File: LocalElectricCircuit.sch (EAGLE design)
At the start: 49 parts, among them IC1 PIC32MX360F512L, U1 ADS1118, U2 ADS1118, X2 MALE_VGA

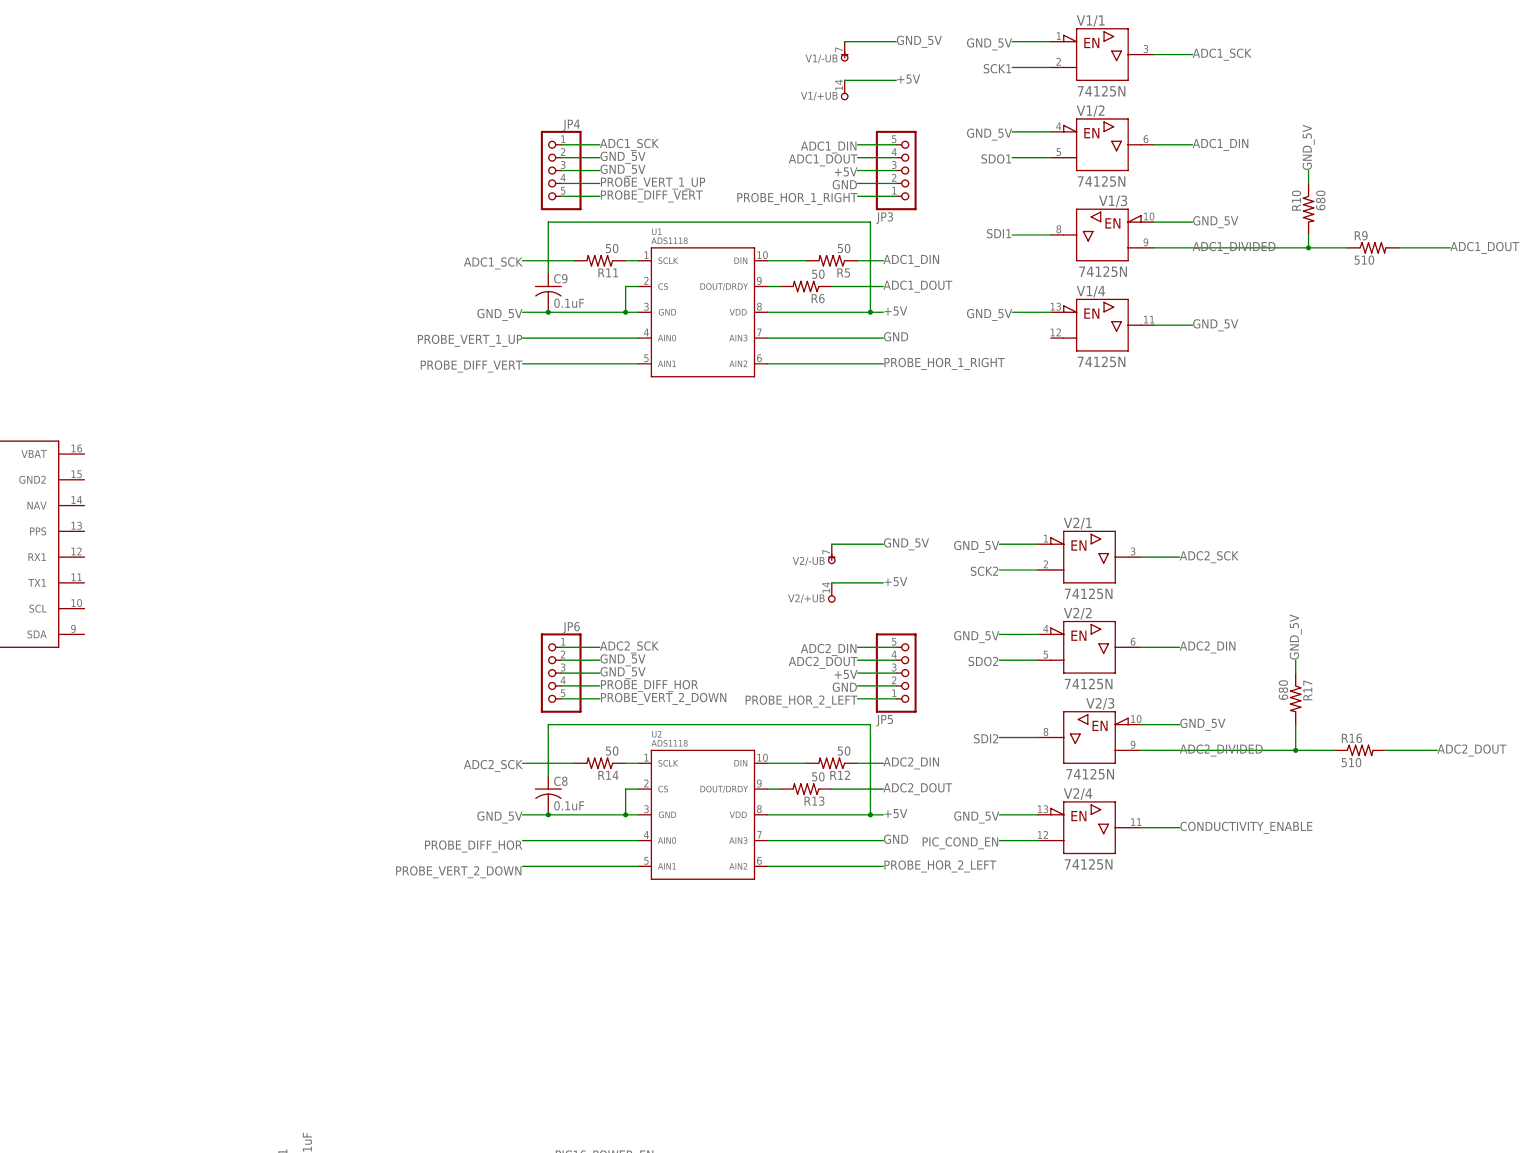
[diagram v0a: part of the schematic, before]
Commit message: Ugh🎈
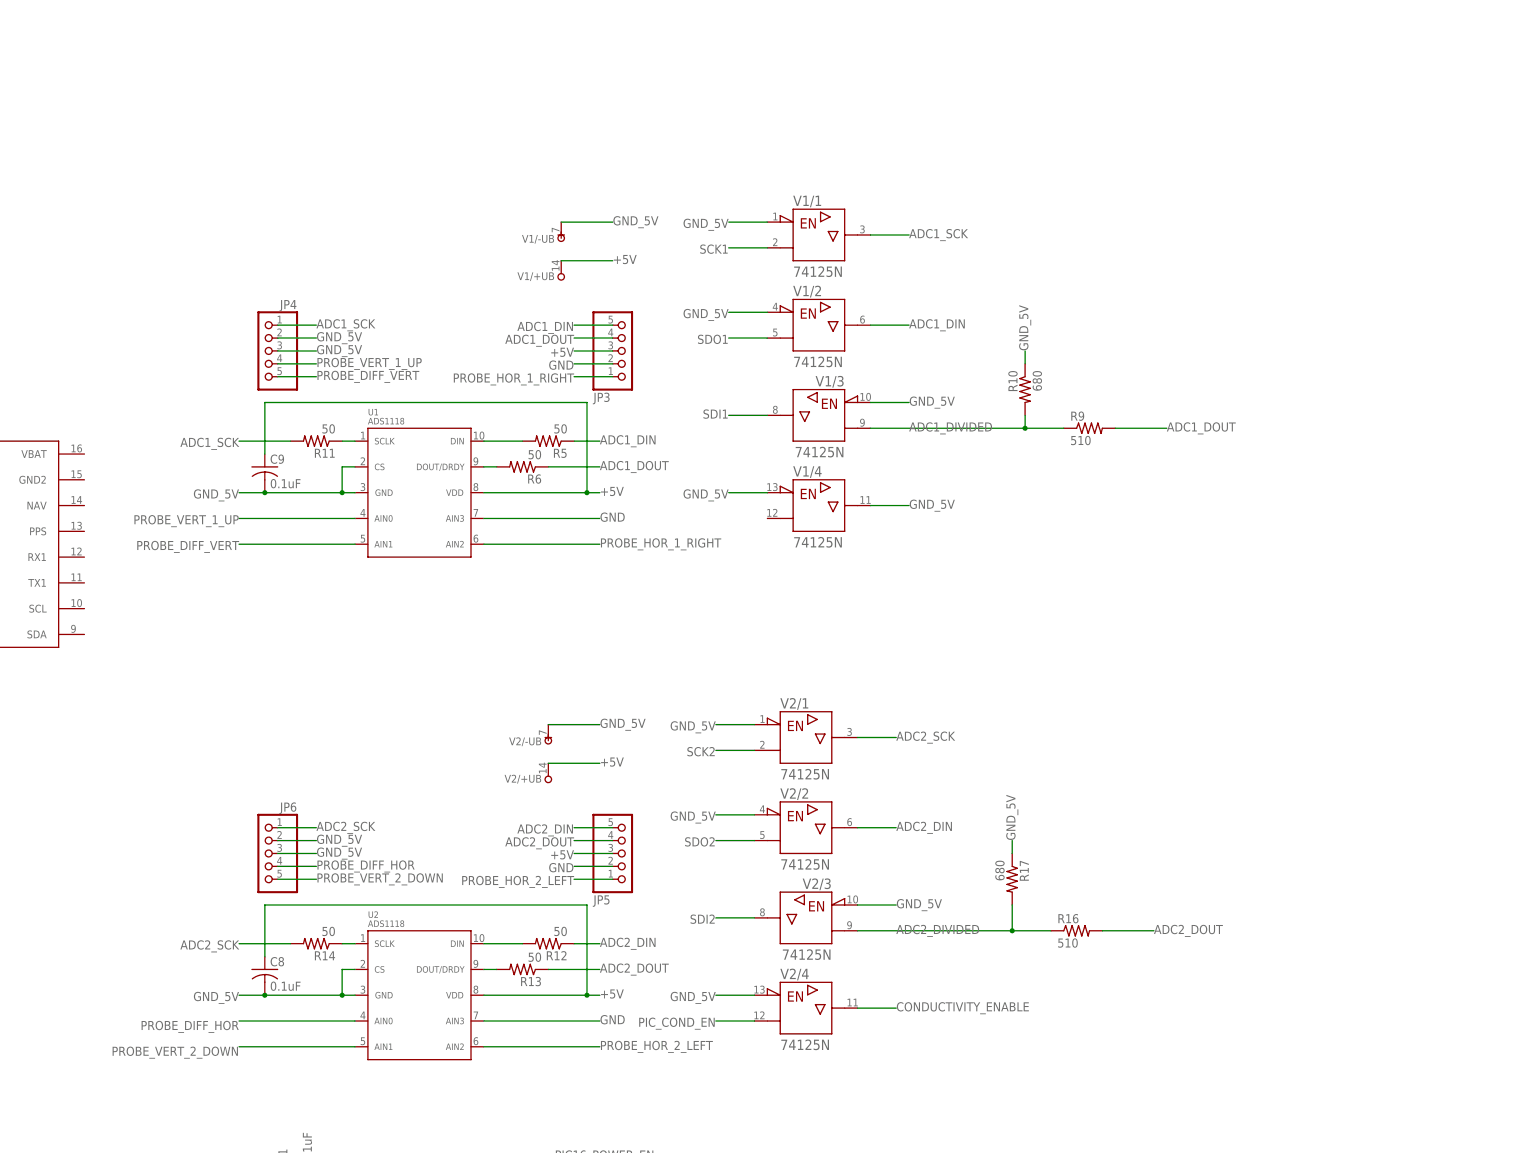
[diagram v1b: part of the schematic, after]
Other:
- moved on the sheet: C8, C9, JP3, JP4, JP5, JP6, R10, R11, R12, R13, R14, R16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
